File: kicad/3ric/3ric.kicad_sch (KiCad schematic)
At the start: 19 parts, among them U1 74LS154, U2 6502-library_65C02S-2, U8 EB6502_isc61c1024-15n

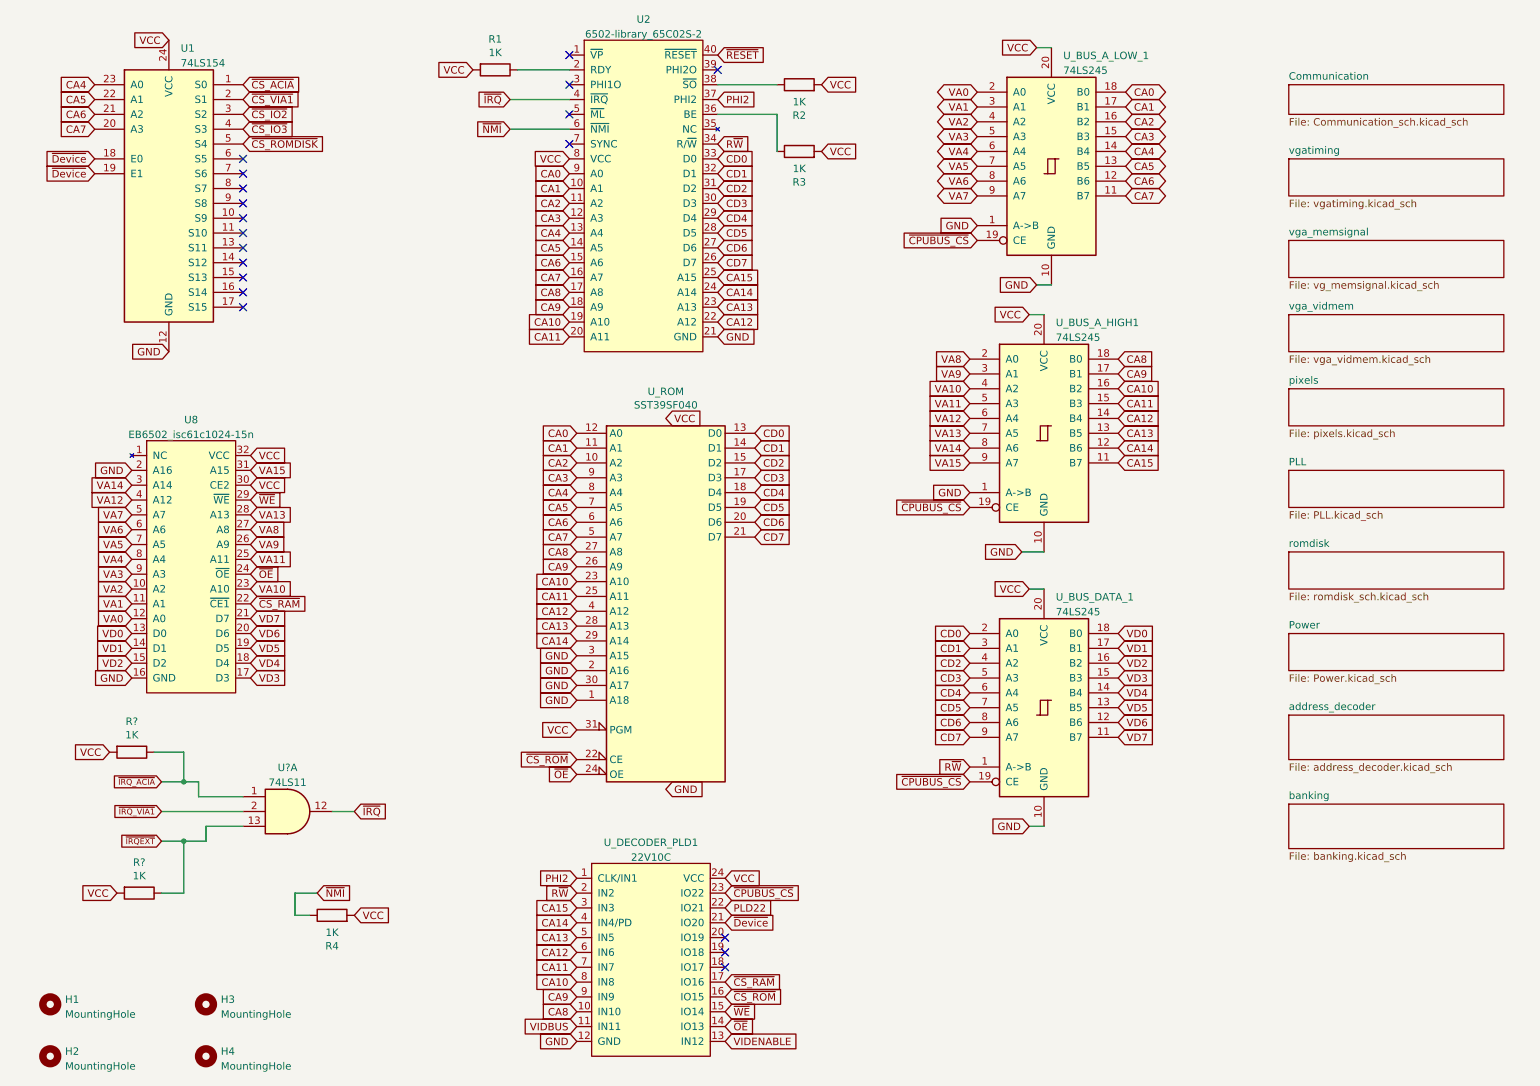
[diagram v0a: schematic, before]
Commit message: updates to logisim project and schematics
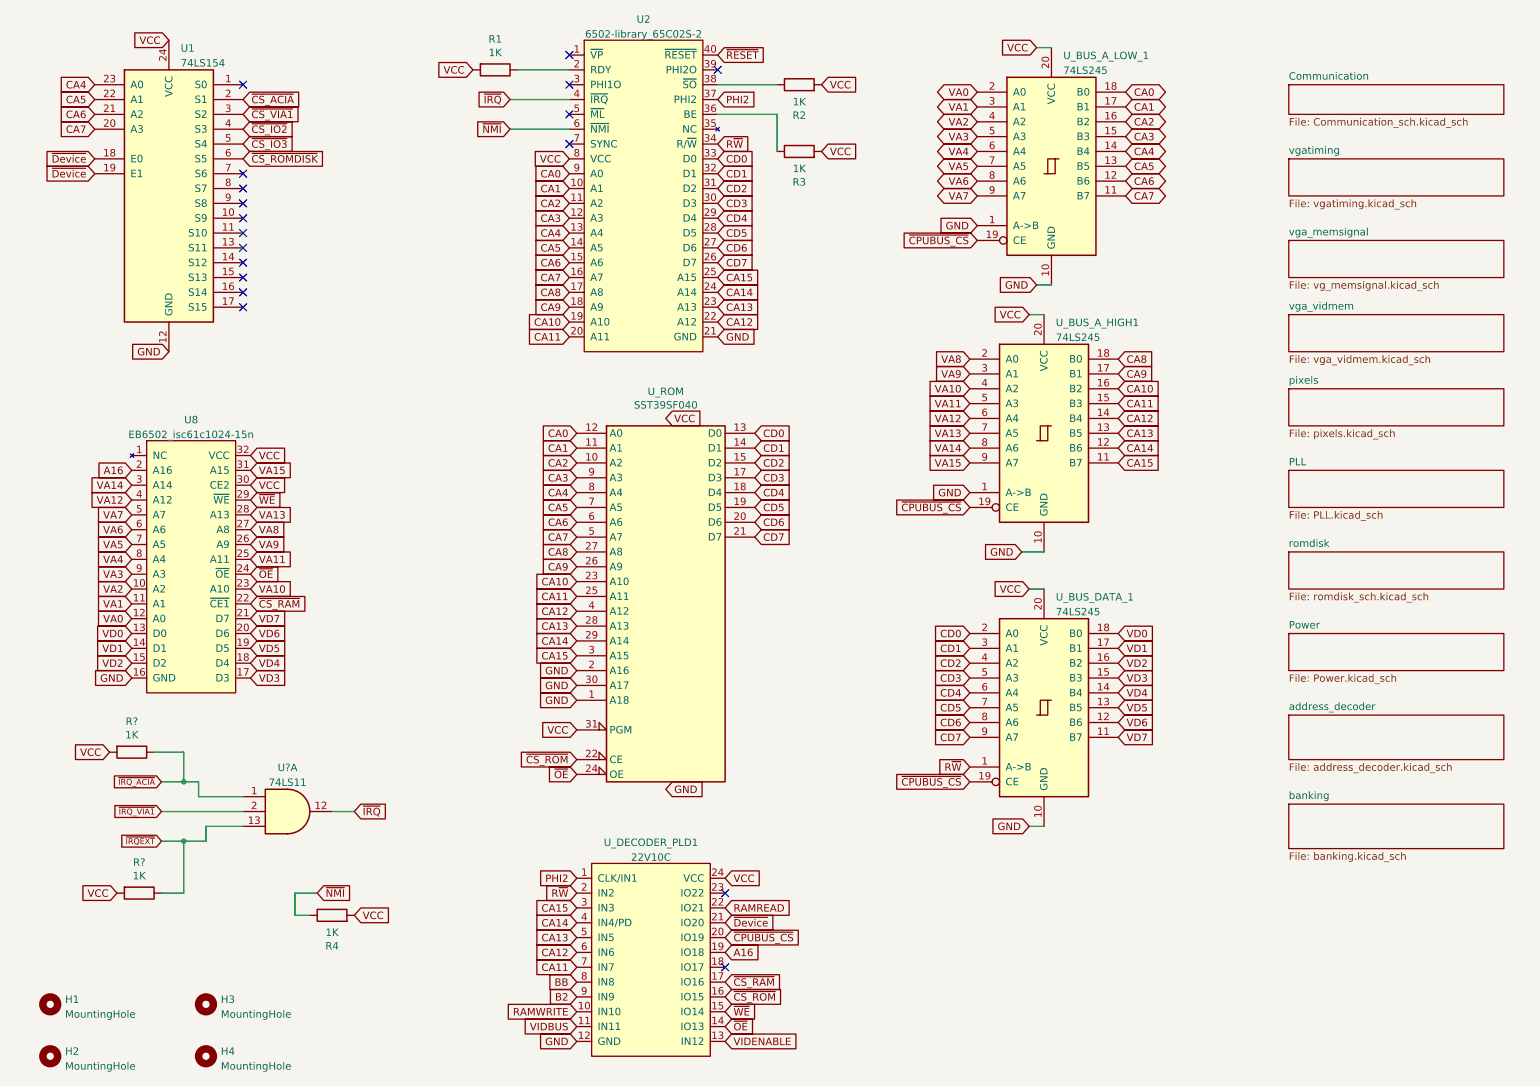
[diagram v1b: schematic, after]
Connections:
- net CA10: no longer U_DECODER_PLD1.8 (IN8)
- net CA15: now also U_ROM.3 (A15)
- net CA8: no longer U_DECODER_PLD1.10 (IN10)
- net CA9: no longer U_DECODER_PLD1.9 (IN9)
- net GND: no longer U8.2 (A16), U_ROM.3 (A15)
- net ~{CPUBUS_CS}: now also U_DECODER_PLD1.20 (IO19); no longer U_DECODER_PLD1.23 (IO22)
- net ~{CS_ACIA}: now also U1.2 (S1); no longer U1.1 (S0)
- net ~{CS_IO2}: now also U1.4 (S3); no longer U1.3 (S2)
- net ~{CS_IO3}: now also U1.5 (S4); no longer U1.4 (S3)
- net ~{CS_ROMDISK}: now also U1.6 (S5); no longer U1.5 (S4)
- net ~{CS_VIA1}: now also U1.3 (S2); no longer U1.2 (S1)
- net A16: now reaches U_DECODER_PLD1.19 (IO18)
- net A16: now also U8.2 (A16)
- net PLD22 renamed RAMREAD
- new net B2: U_DECODER_PLD1.9 (IN9)
- new net BB: U_DECODER_PLD1.8 (IN8)
- new net RAMWRITE: U_DECODER_PLD1.10 (IN10)
- no-connect marks 19 -> 18
